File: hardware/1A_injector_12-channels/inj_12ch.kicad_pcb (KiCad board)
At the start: 2 copper layers, 47 x 58.9 mm, 59 parts, among them M401 CONN_1, P401 CONN_3, P402 CONN_10X2, P403 CONN_16, P404 CONN_1, P405 CONN_1, Q401 OVP_DRIVER, Q402 OVP_DRIVER, Q403 OVP_DRIVER, Q404 OVP_DRIVER, Q405 OVP_DRIVER, Q406 OVP_DRIVER, Q407 OVP_DRIVER, Q408 OVP_DRIVER, Q409 OVP_DRIVER, Q410 OVP_DRIVER, Q411 OVP_DRIVER, Q412 OVP_DRIVER

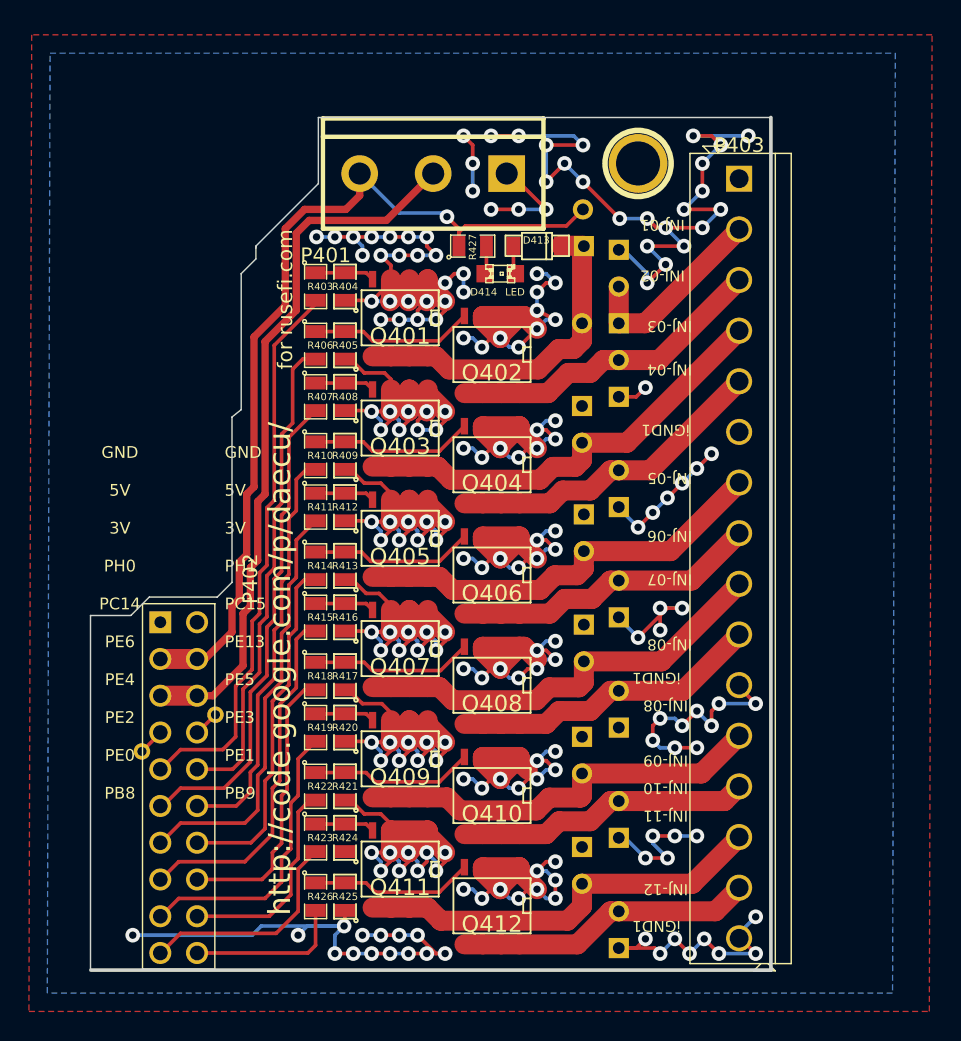
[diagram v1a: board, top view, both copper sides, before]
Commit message: manual sync
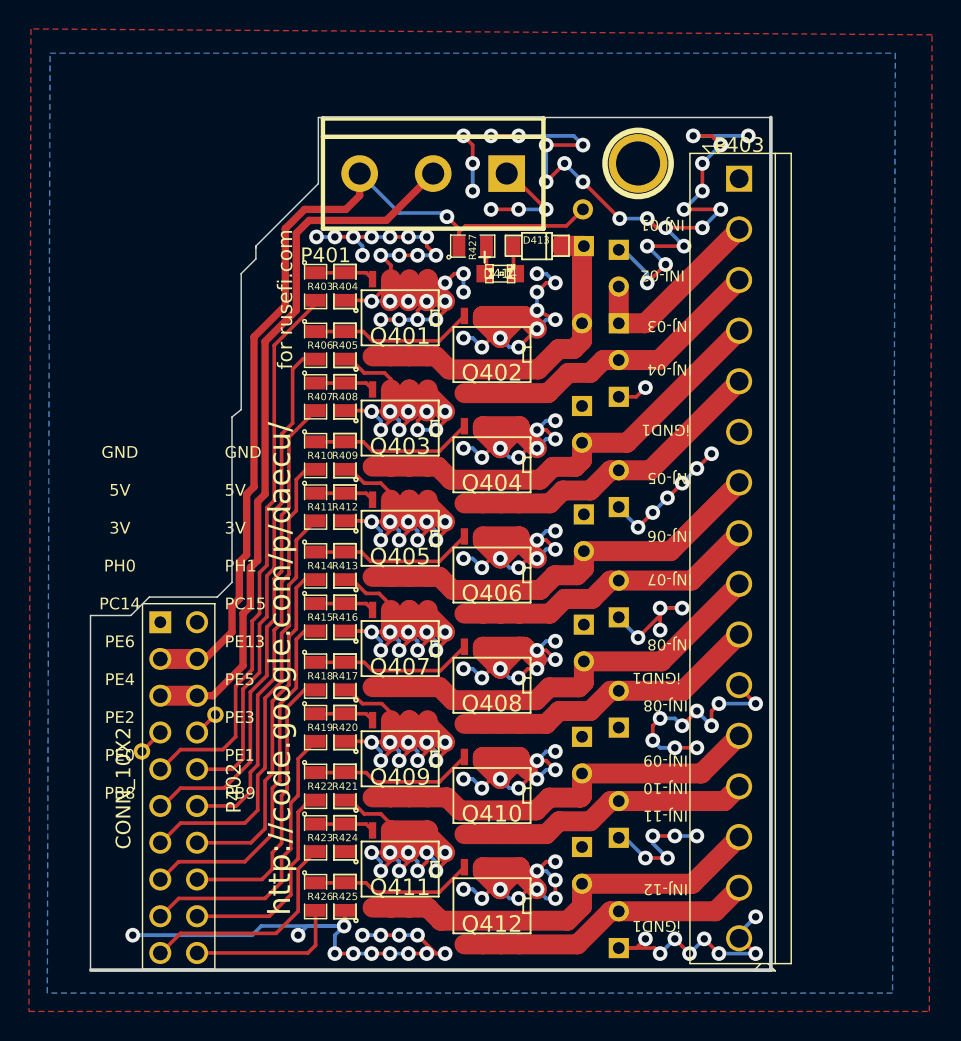
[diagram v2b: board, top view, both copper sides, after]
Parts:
- D414: value LED -> LED_0805; footprint LED-0805 -> LED-0805_A
- P402: footprint pin_array_10x2 -> PIN_ARRAY_10X2_M
